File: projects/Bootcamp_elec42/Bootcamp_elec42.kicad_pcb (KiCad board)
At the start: 2 copper layers, 23.8 x 32 mm, 17 parts, among them SW1 SW_Push

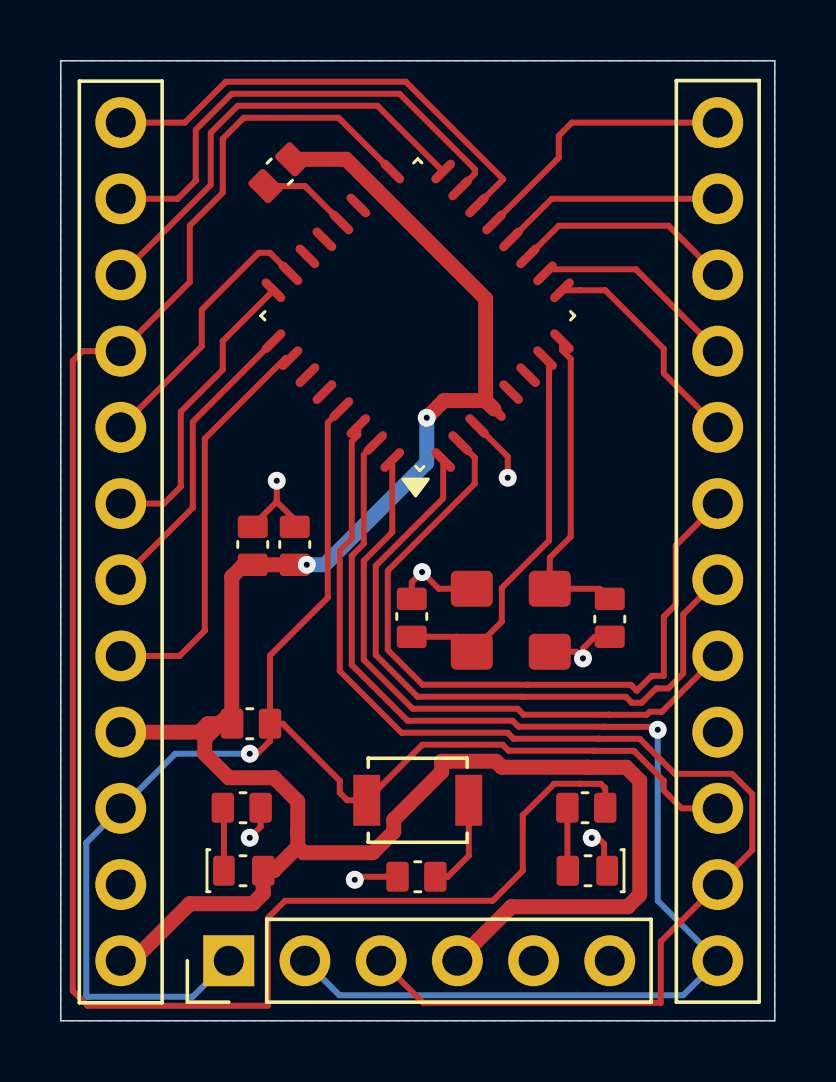
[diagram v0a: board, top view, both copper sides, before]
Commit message: Files needed
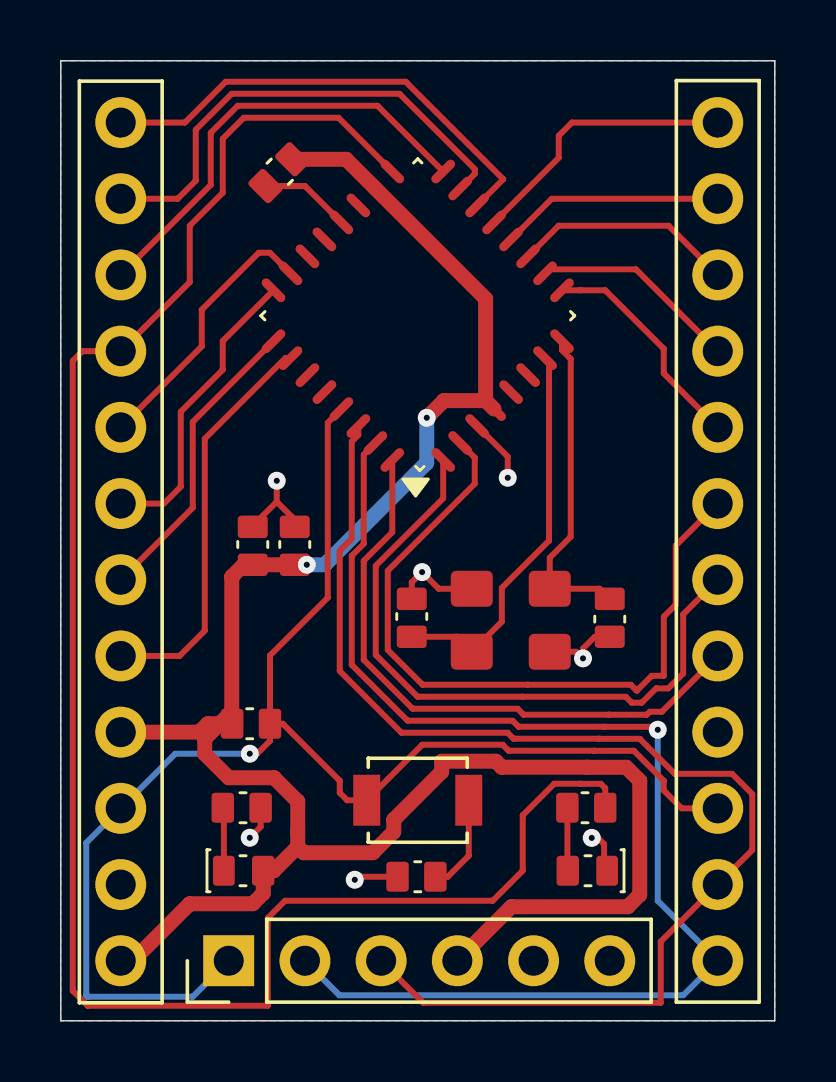
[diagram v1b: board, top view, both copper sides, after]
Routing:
- added copper zone on F.Cu, net (none)
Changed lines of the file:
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@@
 		(tenting front back)
 		(pcbplotparams
-			(layerselection 0x00000000_00000000_55555555_5755f5ff)
-			(plot_on_all_layers_selection 0x00000000_00000000_00000000_00000000)
+			(layerselection 0x00000000_00000000_55555555_5555f5ff)
+			(plot_on_all_layers_selection 0x00000000_00000000_00000000_02000000)
 			(disableapertmacros no)
 			(usegerberextensions no)
@@
 			(plotframeref no)
 			(mode 1)
-			(useauxorigin no)
+			(useauxorigin yes)
 			(hpglpennumber 1)
 			(hpglpenspeed 20)
@@
 			(pdf_back_fp_property_popups yes)
 			(pdf_metadata yes)
-			(pdf_single_document no)
+			(pdf_single_document yes)
 			(dxfpolygonmode yes)
 			(dxfimperialunits yes)
@@
 			(psnegative no)
 			(psa4output no)
-			(plot_black_and_white yes)
+			(plot_black_and_white no)
 			(sketchpadsonfab no)
 			(plotpadnumbers no)
@@
 			(crossoutdnponfab yes)
 			(subtractmaskfromsilk no)
-			(outputformat 1)
+			(outputformat 4)
 			(mirror no)
-			(drillshape 1)
+			(drillshape 0)
 			(scaleselection 1)
 			(outputdirectory "")
@@
 	)
 	(zone
+		(net 0)
+		(net_name "")
+		(layer "F.Cu")
+		(hatch edge 0.5)
+		(connect_pads
+			(clearance 0.5)
+		)
+		(min_thickness 0.25)
+		(filled_areas_thickness no)
+		(fill yes
+			(thermal_gap 0.5)
+			(thermal_bridge_width 0.5)
+			(island_removal_mode 1)
+			(island_area_min 10)
+		)
+		(polygon
+			(pts
+				(xy 135.1 84.5) (xy 158.9 84.5) (xy 158.9 116.5) (xy 135.1 116.5)
+			)
+		)
+	)
+	(zone
